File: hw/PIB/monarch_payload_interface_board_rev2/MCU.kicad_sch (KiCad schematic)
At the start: 29 parts, among them J16 20021121-00008C4LF, SW1 SW_Push, SW2 SW_Push, U2 STM32L4A6VGTx

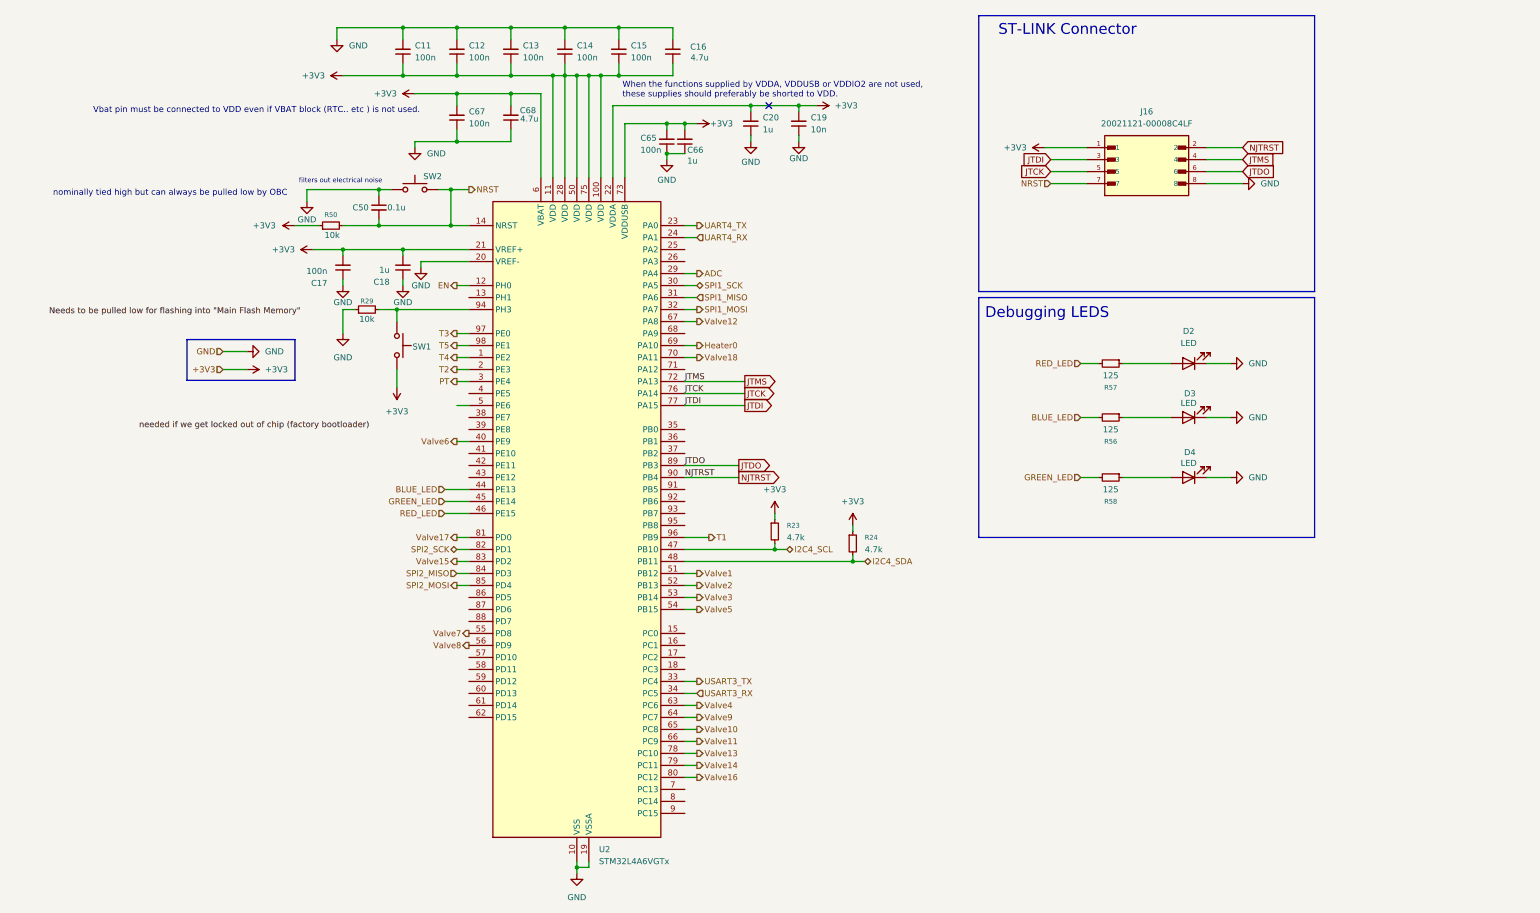
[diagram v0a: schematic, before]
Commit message: Connector Additions
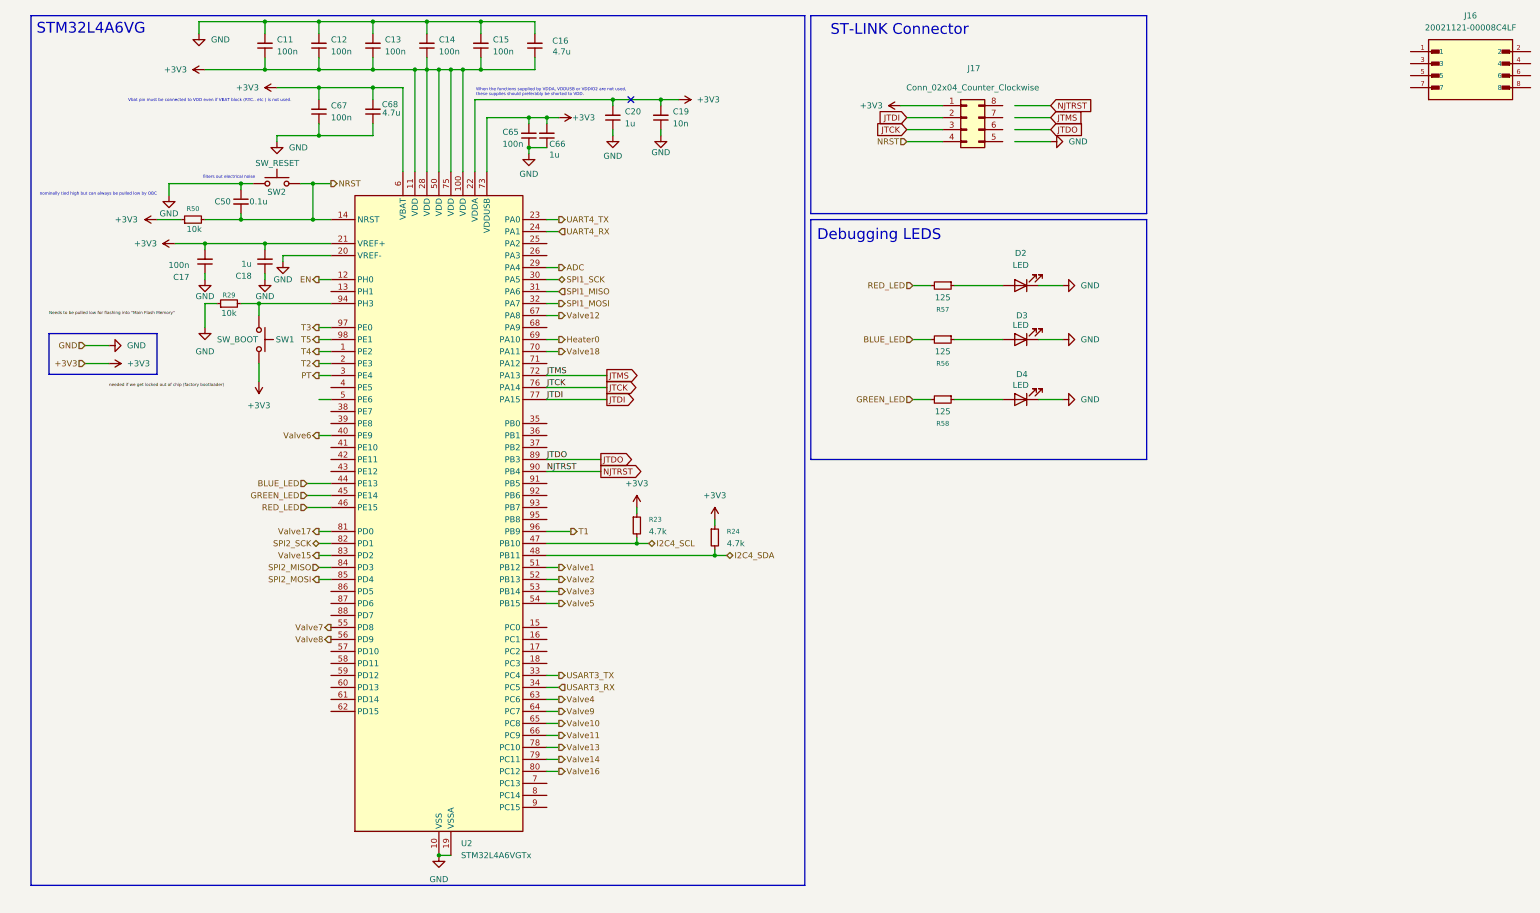
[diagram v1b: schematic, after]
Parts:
- added J17: Conn_02x04_Counter_Clockwise, symbol Connector_Generic:Conn_02x04_Counter_Clockwise
- SW1: value SW_Push -> SW_BOOT
- SW2: value SW_Push -> SW_RESET
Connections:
- net +3V3: now also J17.1 (Pin_1); no longer J16.1
- net GND: no longer J16.8
- net JTCK: now also J17.3 (Pin_3); no longer J16.5
- net JTDI: now also J17.2 (Pin_2); no longer J16.3
- net JTDO: no longer J16.6
- net JTMS: no longer J16.4
- net NJTRST: no longer J16.2
- net NRST: now also J17.4 (Pin_4); no longer J16.7
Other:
- note added: "STM32L4A6VG"
- moved on the sheet: C11, C12, C13, C14, C15, C16, C17, C18, C19, C20, C50, C65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
